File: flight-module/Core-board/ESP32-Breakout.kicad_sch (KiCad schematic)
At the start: 14 parts, among them J3 USB_B_Micro, SW1 SW_MEC_5E, SW2 SW_MEC_5E, U10 ESP32-S3-WROOM-1-N16R2, U9 AZ1084-3.3

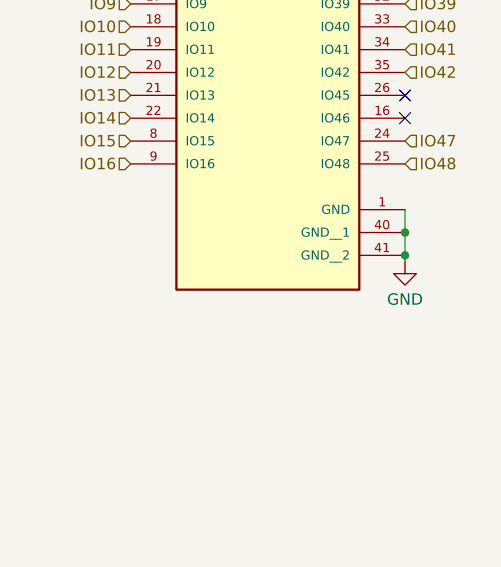
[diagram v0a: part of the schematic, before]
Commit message: Finished flight-core.
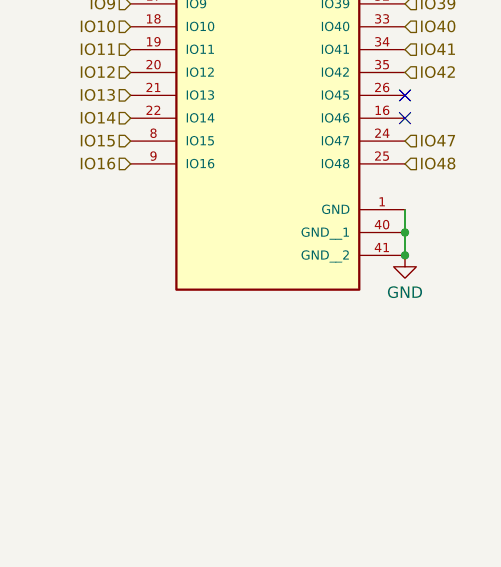
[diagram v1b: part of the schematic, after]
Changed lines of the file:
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@@
-    (stroke (width 0) (type default))
-  )
-  (wire (pts (xy 205.74 99.06) (xy 205.74 99.822))
     (stroke (width 0) (type default))
   )
@@
     )
   )
-  (symbol (lib_id "power:GND") (at 205.74 99.822 0) (mirror y) (unit 1)
-    (in_bom yes) (on_board yes) (dnp no) (fields_autoplaced)
-    (property "Reference" "#PWR01" (at 205.74 106.172 0)
-      (effects (font (size 1.27 1.27)) hide)
-    )
-    (property "Value" "GND" (at 205.74 103.9575 0)
-      (effects (font (size 1.27 1.27)))
-    )
-    (property "Footprint" "" (at 205.74 99.822 0)
-      (effects (font (size 1.27 1.27)) hide)
-    )
-    (property "Datasheet" "" (at 205.74 99.822 0)
-      (effects (font (size 1.27 1.27)) hide)
-    )
+  (symbol (lib_id "power:GND") (at 205.74 99.06 0) (mirror y) (unit 1)
+    (in_bom yes) (on_board yes) (dnp no) (fields_autoplaced)
+    (property "Reference" "#PWR01" (at 205.74 105.41 0)
+      (effects (font (size 1.27 1.27)) hide)
+    )
+    (property "Value" "GND" (at 205.74 103.1955 0)
+      (effects (font (size 1.27 1.27)))
+    )
+    (property "Footprint" "" (at 205.74 99.06 0)
+      (effects (font (size 1.27 1.27)) hide)
+    )
+    (property "Datasheet" "" (at 205.74 99.06 0)
+      (effects (font (size 1.27 1.27)) hide)
+    )

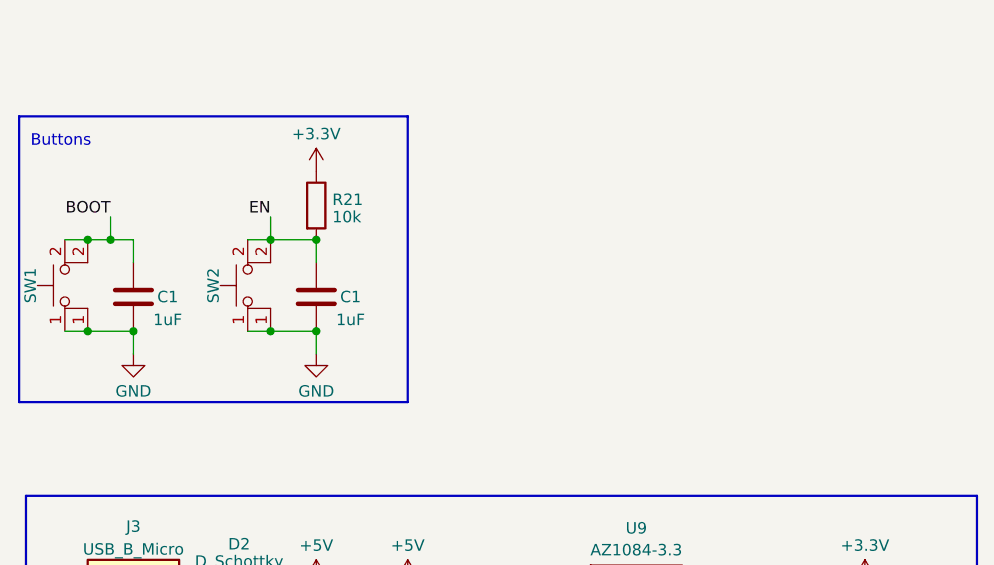
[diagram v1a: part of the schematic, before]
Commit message: Updated core board.
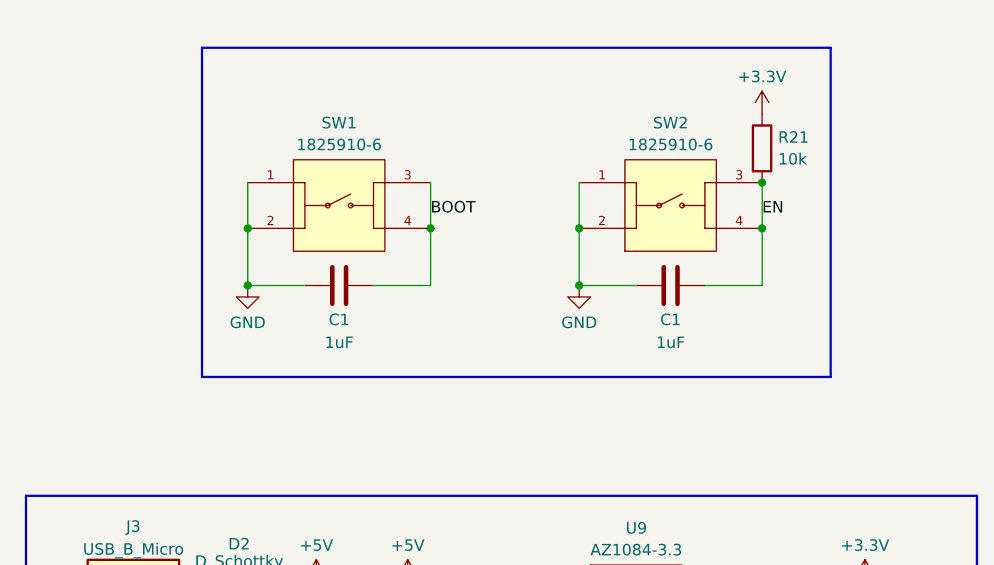
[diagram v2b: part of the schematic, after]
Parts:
- removed C1 (x2): 1uF, Capacitor_SMD:C_0805_2012Metric_Pad1.18x1.45mm_HandSolder, symbol Device:C
- removed SW1, SW2: SW_MEC_5E, Button_Switch_SMD:SW_SPST_TL3305A, symbol Switch:SW_MEC_5E
- added C1 (x2): 1uF, Capacitor_SMD:C_0805_2012Metric_Pad1.18x1.45mm_HandSolder, symbol Device:C
- added SW1, SW2: 1825910-6, 1825910-6:SW_1825910-6-4, symbol 1825910-6:1825910-6
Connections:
- net BOOT: now also C1.2, SW1.3, SW1.4
- net EN: now also C1.2, SW2.3, SW2.4
- net GND: now also C1.1, C1.1, SW1.1, SW1.2, SW2.1, SW2.2
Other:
- note removed: "Buttons"
